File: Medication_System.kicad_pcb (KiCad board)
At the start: 2 copper layers, 43.8 x 38.2 mm, 25 parts, among them J1 USB_C_Receptacle_USB2.0_14P, M1 Motor_Servo, M2 Motor_Servo, M3 Motor_Servo, M4 Motor_Servo, U1 AMS1117-3.3, U2 ESP32-C6-MINI-1, U3 RC1602A-GHW-ESX

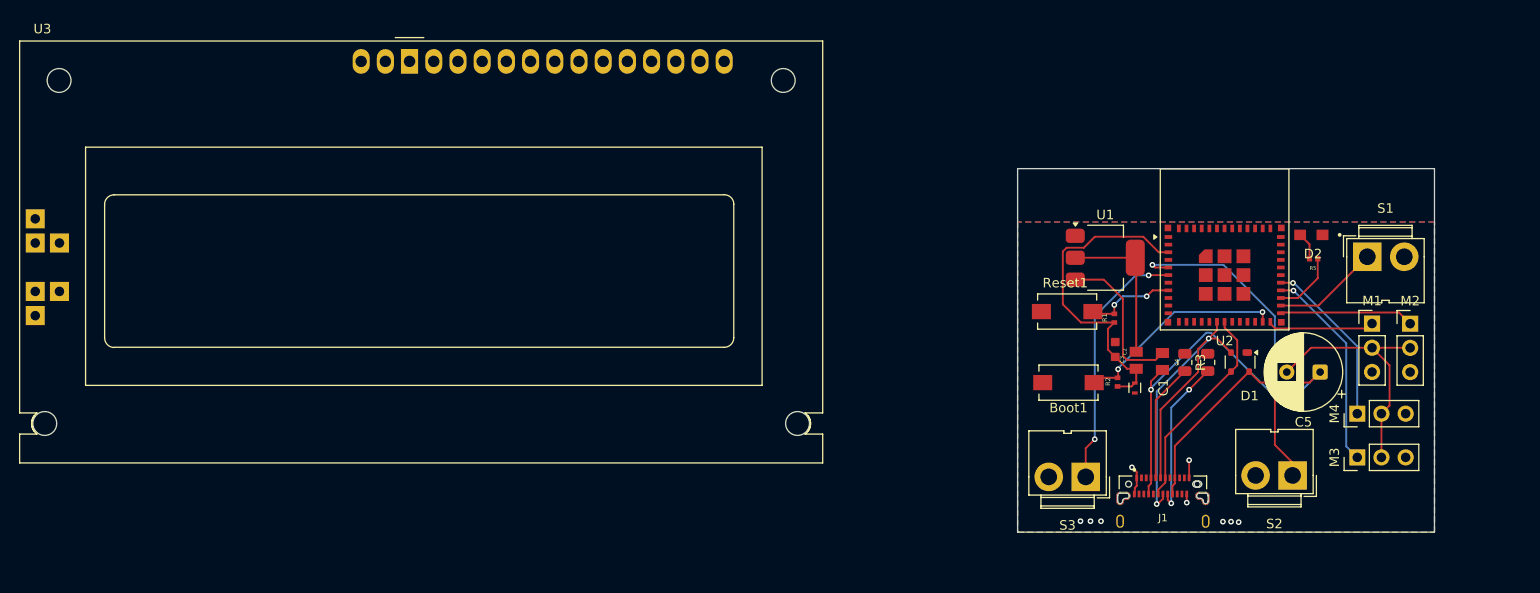
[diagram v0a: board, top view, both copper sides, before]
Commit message: Snapshot of pre-final S3/stepper work before reorganizing
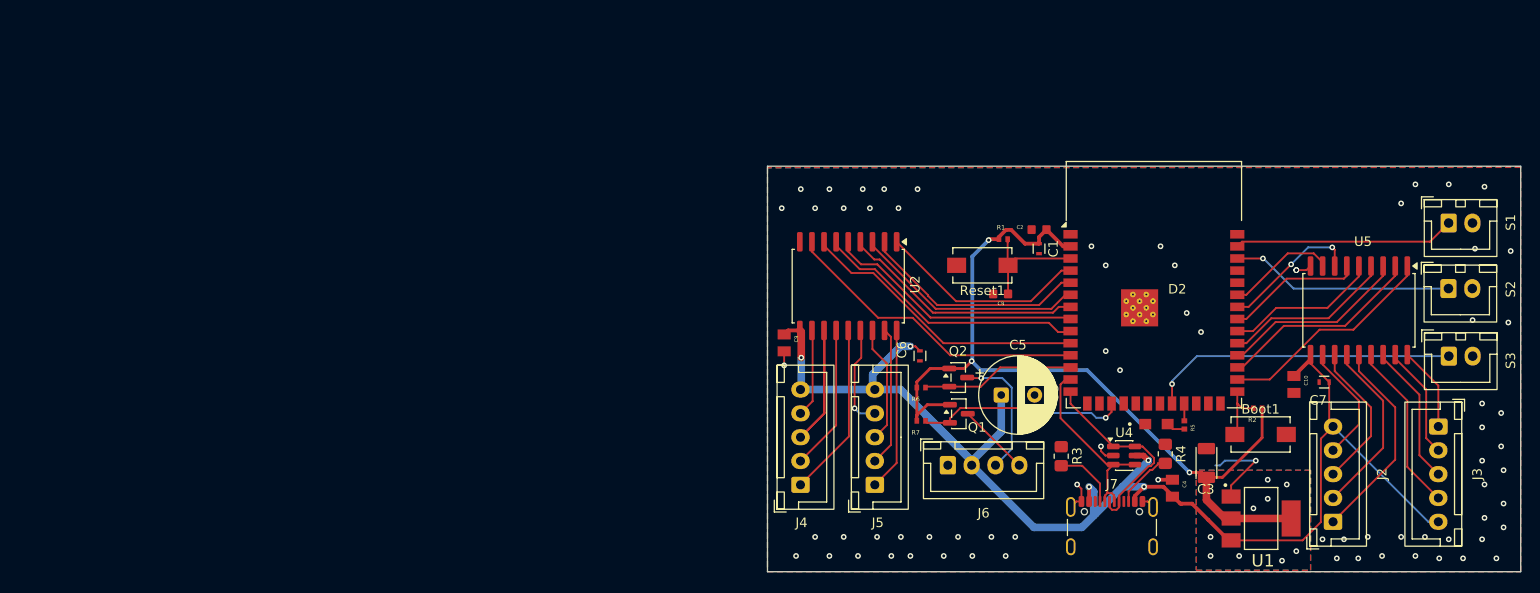
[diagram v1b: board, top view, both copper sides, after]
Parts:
- removed D1: PRTR5V0U2X, Package_TO_SOT_SMD:SOT-143
- removed J1: USB_C_Receptacle_USB2.0_14P, 12401899E412A:AMPHENOL_12401899E412A
- removed M1, M2, M3, M4: Motor_Servo, Connector_PinHeader_2.54mm:PinHeader_1x03_P2.54mm_Vertical
- added C10: GRM21BR61C106KE15L, GRM21BR61C106KE15L:CAPC2012X135N, F.Cu at (172.2, 117.0)
- added C6: CC0402KRX7R7BB104, CC0402KRX7R7BB104:CAPC1005X55N, F.Cu at (133.0, 114.0)
- added C7: CC0402KRX7R7BB104, CC0402KRX7R7BB104:CAPC1005X55N, F.Cu at (175.4, 116.8)
- added C8: CL10A105KO8NNNC, CL10A105KO8NNNC:CAPC1608X90N, F.Cu at (141.5, 107.5)
- added C9: GRM21BR61C106KE15L, GRM21BR61C106KE15L:CAPC2012X135N, F.Cu at (118.8, 112.6)
- added J2: Conn_01x05, Connector_JST:JST_XH_B5B-XH-A_1x05_P2.50mm_Vertical, F.Cu at (176.4, 131.4)
- added J3: Conn_01x05, Connector_JST:JST_XH_B5B-XH-A_1x05_P2.50mm_Vertical, F.Cu at (187.4, 121.4)
- added J4: Conn_01x05, Connector_JST:JST_XH_B5B-XH-A_1x05_P2.50mm_Vertical, F.Cu at (120.5, 127.5)
- added J5: Conn_01x05, Connector_JST:JST_XH_B5B-XH-A_1x05_P2.50mm_Vertical, F.Cu at (128.3, 127.5)
- added J6: Conn_01x04, Connector_JST:JST_XH_B4B-XH-A_1x04_P2.50mm_Vertical, F.Cu at (135.9, 125.5)
- added J7: USB_C_Receptacle_USB2.0_16P, Connector_USB:USB_C_Receptacle_GCT_USB4105-xx-A_16P_TopMnt_Horizontal, F.Cu at (153.1, 133.0)
- added Q1: BSS138, Package_TO_SOT_SMD:SOT-23, F.Cu at (137.1, 120.1)
- added Q2: BSS138, Package_TO_SOT_SMD:SOT-23, F.Cu at (137.0, 116.3)
- added R6: RC0402FR-0710KL, RC0402FR-0710KL:RESC1005X40N, F.Cu at (133.1, 117.3)
- added R7: RC0402FR-0710KL, RC0402FR-0710KL:RESC1005X40N, F.Cu at (133.1, 120.8)
- added U4: USBLC6-2SC6, Package_TO_SOT_SMD:SOT-23-6, F.Cu at (154.4, 124.5)
- added U5: ULN2803A, Package_SO:SOIC-18W_7.5x11.6mm_P1.27mm, F.Cu at (179.1, 109.2)
- C3: value GRM21BR61C106KE15L -> T491A106K016AT; footprint GRM21BR61C106KE15L:CAPC2012X135N -> T491A106K016AT:RESC3216X125N
- R3, R4: footprint Resistor_SMD:R_0805_2012Metric -> Resistor_SMD:R_0805_2012Metric_Pad1.20x1.40mm_HandSolder
- S1, S2, S3: footprint Connector:JWT_A3963_1x02_P3.96mm_Vertical -> Connector_JST:JST_XH_B2B-XH-A_1x02_P2.50mm_Vertical
- U1: value AMS1117-3.3 -> NCP1117LPST33T3G; footprint Package_TO_SOT_SMD:SOT-223-3_TabPin2 -> NCP1117LPST33T3G:SOT230P700X175-4N
- U2: value ESP32-C6-MINI-1 -> ULN2803A; footprint RF_Module:ESP32-C6-MINI-1 -> Package_SO:SOIC-18W_7.5x11.6mm_P1.27mm
- U3: value RC1602A-GHW-ESX -> ESP32-S3-WROOM-1-N8; footprint Display:RC1602A -> RF_Module:ESP32-S3-WROOM-1
- moved U3 81.6 mm to (157.6, 106.5)
- moved S3 40.2 mm to (188.5, 114.0), turned to 0 degrees
- moved U2 39.5 mm to (125.5, 106.7), turned to -90 degrees
- moved C5 33.6 mm to (141.5, 118.1), turned to 0 degrees
- moved U1 31.9 mm to (168.8, 131.1)
- moved D2 25.8 mm to (157.8, 121.2), turned to 0 degrees
- moved S2 25.5 mm to (188.5, 106.9), turned to 0 degrees
- moved R5 22.1 mm to (160.8, 121.2), turned to -90 degrees
- moved Boot1 20.9 mm to (168.8, 122.2), turned to 0 degrees
- moved C1 17.7 mm to (145.5, 102.8), turned to 90 degrees
- moved R3 16.3 mm to (147.8, 124.5)
- moved C2 15.1 mm to (145.5, 100.8), turned to 0 degrees
- moved R2 15.0 mm to (168.5, 119.5), turned to 180 degrees
- moved R1 14.3 mm to (141.8, 101.8), turned to 0 degrees
- moved C4 13.2 mm to (159.5, 127.9)
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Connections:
- Boot1 pad 1: Net-(Boot1-NO) -> /IO0
- C1 pad 1: Net-(U2-3V3) -> GND
- C1 pad 2: GND -> +3V3
- C2 pad 2: Net-(U2-3V3) -> +3V3
- C3 pad 1: Net-(U2-3V3) -> GND
- C3 pad 2: Net-(U1-VO) -> +3V3
- C4 pad 1: Net-(U1-VI) -> GND
- C4 pad 2: Net-(C5-P) -> +5V
- C5 pad 1: Net-(C5-P) -> +5V
- C5 pad 2: Net-(C5-N) -> GND
- R1 pad 1: Net-(U2-3V3) -> +3V3
- R1 pad 2: Net-(Reset1-NO) -> /EN
- R2 pad 1: Net-(U2-3V3) -> +3V3
- R2 pad 2: Net-(Boot1-NO) -> /IO0
- R5 pad 1: Net-(U2-IO21) -> /IO21
- Reset1 pad 1: Net-(Reset1-NO) -> /EN
- S1 pad 1: Net-(S1-Pin_1) -> /IO1
- S2 pad 1: Net-(S2-Pin_1) -> /IO2
- S3 pad 1: Net-(S3-Pin_1) -> /IO14
- U1 pad 2: Net-(U1-VO) -> +3V3
- U1 pad 3: Net-(U1-VI) -> +5V
- U2 pad 1: GND -> /1l1
- U2 pad 10: unconnected-(U2-IO5-Pad10) -> +5V
- U2 pad 11: GND -> Net-(J4-Pin_4)
- U2 pad 12: unconnected-(U2-IO0-Pad12) -> Net-(J4-Pin_3)
- U2 pad 13: unconnected-(U2-IO1-Pad13) -> Net-(J4-Pin_2)
- U2 pad 14: GND -> Net-(J4-Pin_1)
- U2 pad 15: unconnected-(U2-IO6-Pad15) -> Net-(J5-Pin_4)
- U2 pad 16: unconnected-(U2-IO7-Pad16) -> Net-(J5-Pin_3)
- U2 pad 2: GND -> /1l2
- U2 pad 3: Net-(U2-3V3) -> /1l3
- U2 pad 4: unconnected-(U2-NC-Pad4) -> /1l4
- U2 pad 5: Net-(S2-Pin_1) -> /1l5
- U2 pad 6: Net-(S3-Pin_1) -> /1l6
- U2 pad 7: unconnected-(U2-NC-Pad7) -> /1l7
- U2 pad 8: Net-(Reset1-NO) -> /1l8
- U2 pad 9: unconnected-(U2-IO4-Pad9) -> GND
- U3 pad 1: unconnected-(U3-VSS-Pad1) -> GND
- U3 pad 10: unconnected-(U3-DB3-Pad10) -> /1l7
- U3 pad 11: unconnected-(U3-DB4-Pad11) -> /1l8
- U3 pad 12: unconnected-(U3-DB5-Pad12) -> /IO8
- U3 pad 13: unconnected-(U3-DB6-Pad13) -> /D-
- U3 pad 14: unconnected-(U3-DB7-Pad14) -> /D+
- U3 pad 2: unconnected-(U3-VDD-Pad2) -> +3V3
- U3 pad 3: unconnected-(U3-Vo-Pad3) -> /EN
- U3 pad 4: unconnected-(U3-RS-Pad4) -> /1l1
- U3 pad 5: unconnected-(U3-R/~{W}-Pad5) -> /1l2
- U3 pad 6: unconnected-(U3-~{E}-Pad6) -> /1l3
- U3 pad 7: unconnected-(U3-DB0-Pad7) -> /1l4
- U3 pad 8: unconnected-(U3-DB1-Pad8) -> /1l5
- U3 pad 9: unconnected-(U3-DB2-Pad9) -> /1l6
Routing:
- net +5V: track 0.00 -> 157.9 mm, vias 0 -> 5
- net +3V3: track 0.00 -> 92.7 mm, vias 0 -> 12
- net Net-(C5-P): track 62.1 -> 0.00 mm, vias 1 -> 0
- net Net-(C5-N): track 37.9 -> 0.00 mm
- net Net-(U2-3V3): track 34.6 -> 0.00 mm
- net Net-(S2-Pin_1): track 34.3 -> 0.00 mm, vias 2 -> 0
- net /1l8: track 0.00 -> 32.7 mm
- net /IO14: track 0.00 -> 32.6 mm, vias 0 -> 1
- net /1l7: track 0.00 -> 30.5 mm
- net /1l6: track 0.00 -> 28.8 mm
- net Net-(J5-Pin_2): track 42.8 -> 15.0 mm, vias 2 -> 0
- net /1l5: track 0.00 -> 27.3 mm
- net Net-(S3-Pin_1): track 26.8 -> 0.00 mm, vias 2 -> 0
- net /1l4: track 0.00 -> 26.5 mm
- net /1l3: track 0.00 -> 24.5 mm
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- added copper zone on B.Cu, net +3V3
- added copper zone on F.Cu, net +3V3
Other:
- board size 43.8 x 38.2 mm -> 79.1 x 42.6 mm
